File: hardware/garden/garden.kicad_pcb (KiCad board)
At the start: 4 copper layers, 53.3 x 83.8 mm, 53 parts, among them J1 CONN_01X40, J2 CONN_01X08, J3 CONN_01X06, J4 CONN_01X10, J5 CONN_01X08, J7 Micro_SD_Card_CD, J8 CONN_01X13, J9 CONN_01X06, M1 ESP-11, M2 CONN_01X01, M3 CONN_01X01, M4 CONN_01X01, M5 CONN_01X01, P1 USB_OTG, Q1 Q_NMOS_GSD, SW1 RESET, SW2 BOOT, U1 AZ1117-3.3, U2 STM32F745ZETx, U3 IS42S16160G, Y1 12MHz

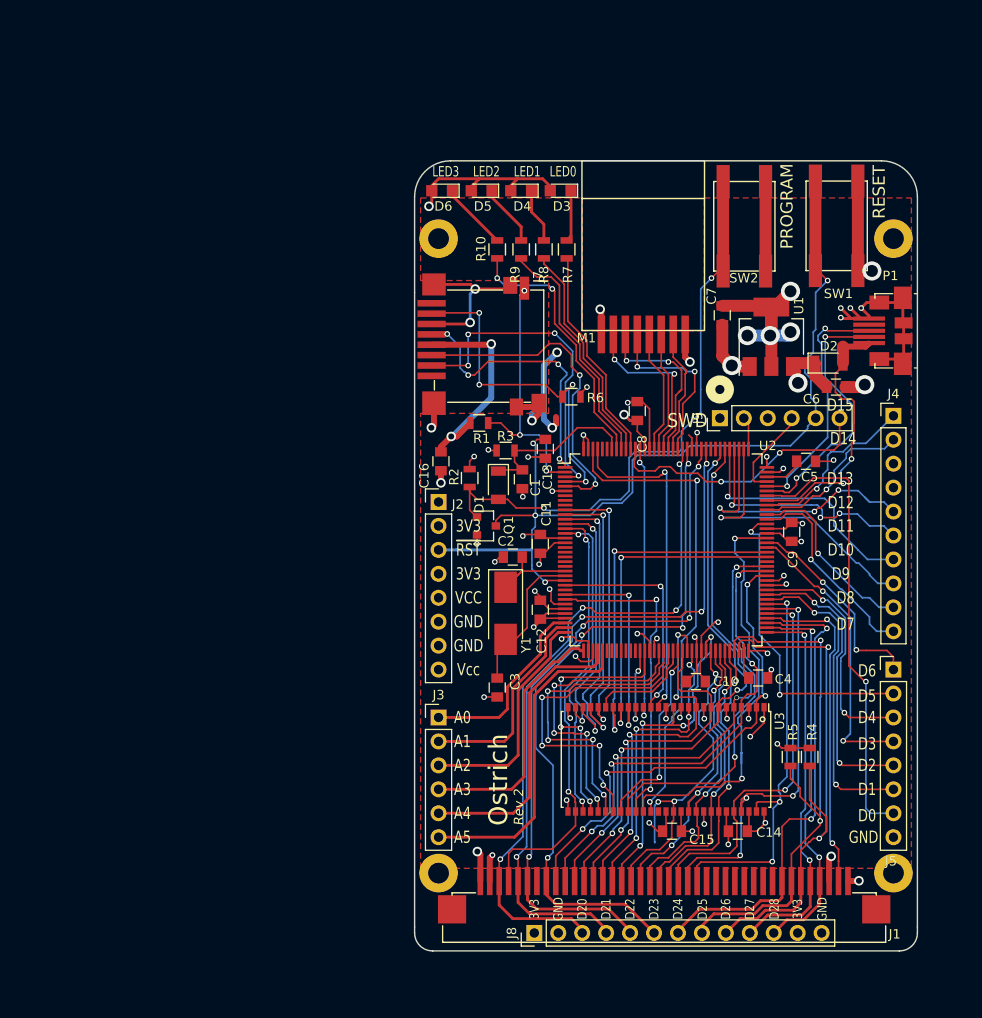
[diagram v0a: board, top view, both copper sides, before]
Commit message: Designed garden controller
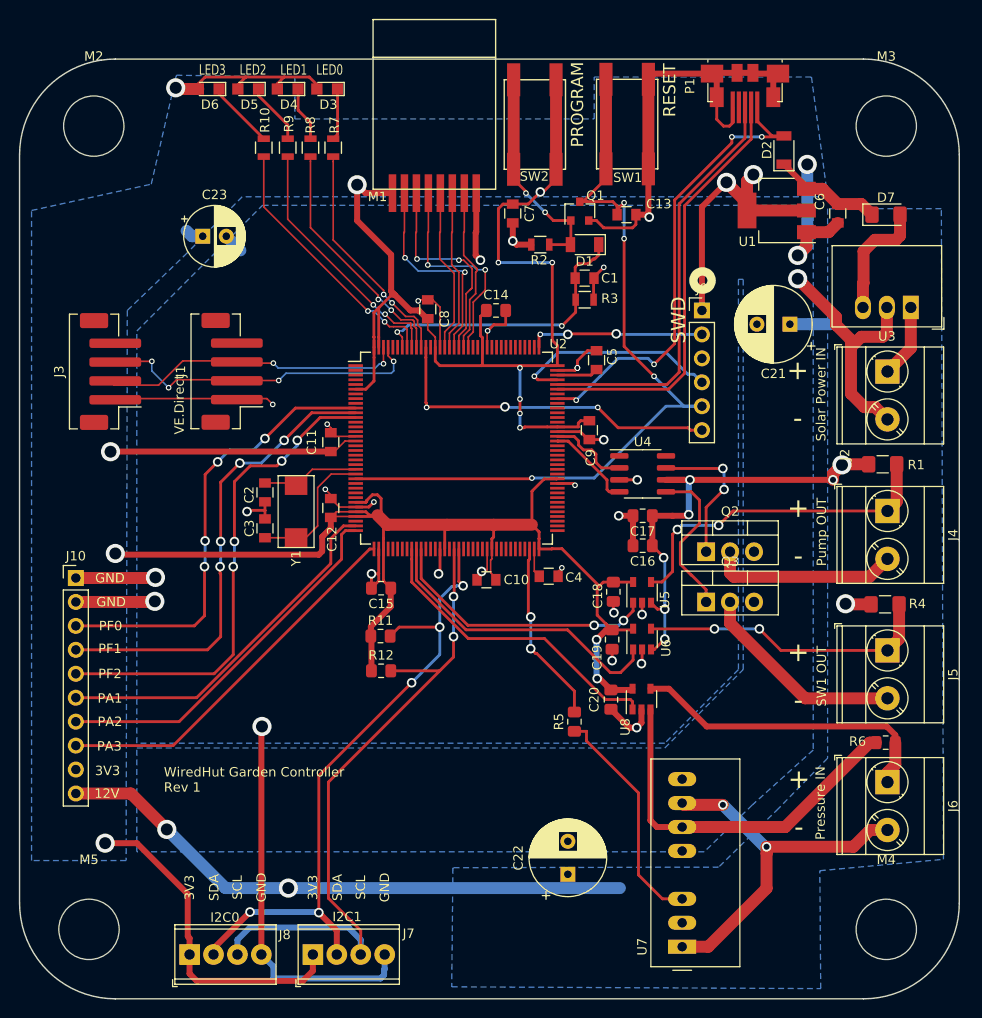
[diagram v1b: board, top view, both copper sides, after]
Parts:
- added C17: 1uF, Capacitor_SMD:C_0805_2012Metric_Pad1.15x1.40mm_HandSolder, F.Cu at (122.0, 98.0)
- added C18: 0.1uF, Capacitor_SMD:C_0805_2012Metric_Pad1.15x1.40mm_HandSolder, F.Cu at (118.9, 106.0)
- added C19: 0.1uF, Capacitor_SMD:C_0805_2012Metric_Pad1.15x1.40mm_HandSolder, F.Cu at (118.7, 111.1)
- added C20: 0.1uF, Capacitor_SMD:C_0805_2012Metric_Pad1.15x1.40mm_HandSolder, F.Cu at (118.6, 117.5)
- added C21: 220uF, Capacitor_THT:CP_Radial_D8.0mm_P3.50mm, F.Cu at (137.6, 77.7)
- added C22: 220uF, Capacitor_THT:CP_Radial_D8.0mm_P3.50mm, F.Cu at (114.0, 136.0)
- added C23: 22uF, Capacitor_THT:CP_Radial_D6.3mm_P2.50mm, F.Cu at (75.3, 68.3)
- added D7: D_Schottky, Diode_SMD:D_1206_3216Metric_Pad1.42x1.75mm_HandSolder, F.Cu at (147.8, 66.0)
- added J10: CONN_01X10, Connector_PinHeader_2.54mm:PinHeader_1x10_P2.54mm_Vertical, F.Cu at (61.8, 104.6)
- added J6: CONN_01X02, TerminalBlock_Phoenix:TerminalBlock_Phoenix_MKDS-3-2-5.08_1x02_P5.08mm_Horizontal, F.Cu at (148.0, 126.2)
- added Q2: Q_NMOS_GDS, Package_TO_SOT_THT:TO-220-3_Vertical, F.Cu at (128.7, 101.8)
- added Q3: Q_NMOS_GDS, Package_TO_SOT_THT:TO-220-3_Vertical, F.Cu at (128.7, 107.1)
- added R11: 1kR, Resistor_SMD:R_0805_2012Metric_Pad1.15x1.40mm_HandSolder, F.Cu at (94.2, 110.7)
- added R12: 1kR, Resistor_SMD:R_0805_2012Metric_Pad1.15x1.40mm_HandSolder, F.Cu at (94.2, 114.4)
- added U4: MIC4427, Package_SO:SOIC-8_3.9x4.9mm_P1.27mm, F.Cu at (122.0, 93.5)
- added U5: INA193, Package_TO_SOT_SMD:SOT-23-5, F.Cu at (121.9, 106.1)
- added U6: INA193, Package_TO_SOT_SMD:SOT-23-5, F.Cu at (121.9, 111.1)
- added U7: TEC2-1215WI, Converter_DCDC:Converter_DCDC_TRACO_TMR-xxxx_THT, F.Cu at (126.2, 143.7)
- added U8: INA193, Package_TO_SOT_SMD:SOT-23-5, F.Cu at (121.9, 117.4)
- C14: footprint Capacitors_SMD:C_0805 -> Capacitor_SMD:C_0805_2012Metric_Pad1.15x1.40mm_HandSolder
- C15, C16: value 10uF -> 0.1uF; footprint Capacitors_SMD:C_0805 -> Capacitor_SMD:C_0805_2012Metric_Pad1.15x1.40mm_HandSolder
- J1: value CONN_01X40 -> CONN_01X04; footprint ER-CON40HB-2:ER-CON40HB-2 -> Connector_JST:JST_PH_B4B-PH-SM4-TB_1x04-1MP_P2.00mm_Vertical
- J2, J5: value CONN_01X08 -> CONN_01X02; footprint Pin_Headers:Pin_Header_Straight_1x08_Pitch2.54mm -> TerminalBlock_Phoenix:TerminalBlock_Phoenix_MKDS-3-2-5.08_1x02_P5.08mm_Horizontal
- J3: value CONN_01X06 -> CONN_01X04; footprint Pin_Headers:Pin_Header_Straight_1x06_Pitch2.54mm -> Connector_JST:JST_PH_B4B-PH-SM4-TB_1x04-1MP_P2.00mm_Vertical
- J4: value CONN_01X10 -> CONN_01X02; footprint Connector_PinHeader_2.54mm:PinHeader_1x10_P2.54mm_Vertical -> TerminalBlock_Phoenix:TerminalBlock_Phoenix_MKDS-3-2-5.08_1x02_P5.08mm_Horizontal
- J7: value Micro_SD_Card_CD -> CONN_01X04; footprint Amphenol:Amphenol_1140084168 -> TerminalBlock_Phoenix:TerminalBlock_Phoenix_MPT-0,5-4-2.54_1x04_P2.54mm_Horizontal
- J8: value CONN_01X13 -> CONN_01X04; footprint Pin_Headers:Pin_Header_Straight_1x13_Pitch2.54mm -> TerminalBlock_Phoenix:TerminalBlock_Phoenix_MPT-0,5-4-2.54_1x04_P2.54mm_Horizontal
- M2, M3, M4, M5: footprint Mechanical:M2_HOLE -> MountingHole:MountingHole_6.4mm_M6
- R1, R4: value 10KR -> 10mR; footprint Resistors_SMD:R_0805 -> Resistor_SMD:R_1206_3216Metric_Pad1.42x1.75mm_HandSolder
- R5: value 10KR -> 1kR; footprint Resistors_SMD:R_0805 -> Resistor_SMD:R_0805_2012Metric_Pad1.15x1.40mm_HandSolder
- R6: value 10KR -> 6.8R; footprint Resistors_SMD:R_0805 -> Resistor_SMD:R_0805_2012Metric_Pad1.15x1.40mm_HandSolder
- U1: footprint SOT-223 -> Package_TO_SOT_SMD:SOT-223
- U3: value IS42S16160G -> R-78B5.0-2.0; footprint TSOPII:TSOPII-54_10.16x22.22mm-Pitch0.8mm -> Converter_DCDC:Converter_DCDC_RECOM_R-78B-2.0_THT
- moved J1 85.4 mm to (78.4, 82.7), turned to 90 degrees
- moved J7 70.5 mm to (87.0, 144.5), turned to 0 degrees
- moved C14 60.9 mm to (106.4, 76.2)
- moved U3 54.5 mm to (150.4, 75.9), turned to 180 degrees
- moved J3 50.6 mm to (65.5, 82.7), turned to 90 degrees
- moved J2 49.6 mm to (148.0, 82.7), turned to 270 degrees
- moved R6 49.6 mm to (147.8, 122.0)
- moved R1 43.0 mm to (147.4, 92.5)
- moved C15 40.2 mm to (94.2, 105.7)
- moved M2 38.5 mm to (63.8, 56.6)
- moved M5 37.6 mm to (63.2, 141.9)
- moved J8 36.6 mm to (73.9, 144.5), turned to 0 degrees
- moved Q1 34.8 mm to (115.3, 65.7), turned to 90 degrees
- moved P1 30.3 mm to (132.8, 52.3), turned to 270 degrees
- moved C3 29.9 mm to (81.9, 99.3), turned to 90 degrees
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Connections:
- net /PA9 renamed /Vusb
- C16 pad 1: +3V3 -> +12V
- J1 pad 2: /LCD_BL -> /VD_RX
- J1 pad 3: GND -> /VD_TX
- J1 pad 4: /TOUCH_WAKE -> (no net)
- J2 pad 1: Net-(J2-Pad1) -> +12V
- J2 pad 2: +3V3 -> GND
- J3 pad 1: /PA0 -> GND
- J3 pad 2: /PA1 -> /VD_TX
- J3 pad 3: /PA2 -> /VD_RX
- J3 pad 4: /PA3 -> (no net)
- J4 pad 1: /PA8 -> Net-(J4-Pad1)
- J4 pad 2: /PC9 -> Net-(J4-Pad2)
- J5 pad 1: /PG7 -> Net-(J5-Pad1)
- J5 pad 2: /PC6 -> Net-(J5-Pad2)
- J7 pad 1: Net-(J7-Pad1) -> +3V3
- J7 pad 2: /SD_CS -> /SDA
- J7 pad 3: /SD_MOSI -> /SCL
- J7 pad 4: +3V3 -> GND
- J8 pad 2: GND -> /SDA
- J8 pad 3: /~LCD_CS -> /SCL
- J8 pad 4: /~LCD_RD -> GND
- M2 pad 1: Net-(M2-Pad1) -> (no net)
- M3 pad 1: Net-(M3-Pad1) -> (no net)
- M4 pad 1: Net-(M4-Pad1) -> (no net)
- M5 pad 1: Net-(M5-Pad1) -> (no net)
- P1 pad 4: Net-(P1-Pad4) -> (no net)
- R1 pad 1: +3V3 -> +12V
- R1 pad 2: /SD_CD -> Net-(J4-Pad1)
- R4 pad 1: +3V3 -> +12V
- R4 pad 2: /TOUCH_SDA -> Net-(J5-Pad1)
- R5 pad 1: +3V3 -> Net-(R5-Pad1)
- R5 pad 2: /TOUCH_SCL -> /PRESSURE_PWR
- R6 pad 1: +3V3 -> Net-(J6-Pad1)
- R6 pad 2: /SD_MISO -> Net-(R6-Pad2)
- U2 pad 1: /SD_SCLK -> (no net)
- U2 pad 10: /A0 -> /PF0
- U2 pad 100: /PA8 -> (no net)
- U2 pad 102: /PA10 -> (no net)
- U2 pad 11: /A1 -> /PF1
- U2 pad 110: /PA15 -> (no net)
- U2 pad 111: /PC10 -> (no net)
- U2 pad 112: /PC11 -> (no net)
- U2 pad 113: /PC12 -> (no net)
- U2 pad 114: /D2 -> (no net)
- U2 pad 115: /D3 -> (no net)
- U2 pad 116: Net-(U2-Pad116) -> (no net)
- U2 pad 117: Net-(U2-Pad117) -> (no net)
- U2 pad 118: /~LCD_RD -> (no net)
- U2 pad 119: /~LCD_WR -> (no net)
- U2 pad 12: /A2 -> /PF2
- U2 pad 122: /LCD_TE -> (no net)
- U2 pad 123: /~LCD_CS -> (no net)
- U2 pad 13: /A3 -> (no net)
- U2 pad 132: /SDNCAS -> (no net)
- U2 pad 139: Net-(U2-Pad139) -> (no net)
- U2 pad 14: /A4 -> (no net)
- U2 pad 140: Net-(U2-Pad140) -> (no net)
- U2 pad 141: /NBL0 -> /VD_RX
- U2 pad 142: /NBL1 -> /VD_TX
- U2 pad 15: /A5 -> (no net)
- U2 pad 18: Net-(U2-Pad18) -> (no net)
- U2 pad 19: Net-(U2-Pad19) -> (no net)
- U2 pad 2: /SD_CD -> (no net)
- U2 pad 20: Net-(U2-Pad20) -> (no net)
- U2 pad 21: Net-(U2-Pad21) -> (no net)
- U2 pad 22: Net-(U2-Pad22) -> (no net)
- U2 pad 26: /SDNWE -> (no net)
- U2 pad 27: Net-(U2-Pad27) -> (no net)
- U2 pad 28: /SDNE0 -> (no net)
- U2 pad 29: /SDCKE0 -> (no net)
- U2 pad 3: /SD_CS -> (no net)
- U2 pad 34: /PA0 -> (no net)
- U2 pad 4: /SD_MISO -> (no net)
- U2 pad 40: /PA4 -> (no net)
- U2 pad 41: /PA5 -> (no net)
- U2 pad 42: Net-(U2-Pad42) -> (no net)
- U2 pad 43: /PA7 -> (no net)
- U2 pad 44: Net-(U2-Pad44) -> (no net)
- U2 pad 45: Net-(U2-Pad45) -> /PRESSURE_CUR
- U2 pad 46: Net-(U2-Pad46) -> /SW1_CUR
- U2 pad 47: Net-(U2-Pad47) -> /SW0_CUR
- U2 pad 48: Net-(U2-Pad48) -> (no net)
- U2 pad 49: /SDNRAS -> (no net)
- U2 pad 5: /SD_MOSI -> (no net)
- U2 pad 50: /A6 -> (no net)
- U2 pad 53: /A7 -> (no net)
- U2 pad 54: /A8 -> /SCL
- U2 pad 55: /A9 -> /SDA
- U2 pad 56: /A10 -> (no net)
- U2 pad 57: /A11 -> (no net)
- U2 pad 58: /D4 -> (no net)
- U2 pad 59: /D5 -> (no net)
- U2 pad 60: /D6 -> (no net)
- U2 pad 63: /D7 -> (no net)
- U2 pad 64: /D8 -> (no net)
- U2 pad 65: /D9 -> (no net)
- U2 pad 66: /D10 -> (no net)
- U2 pad 67: /D11 -> (no net)
- U2 pad 68: /D12 -> (no net)
- U2 pad 69: /TOUCH_SCL -> (no net)
- U2 pad 7: Net-(U2-Pad7) -> (no net)
- U2 pad 70: /TOUCH_SDA -> /PRESSURE_PWR
- U2 pad 73: /TOUCH_INT -> (no net)
- U2 pad 74: /TOUCH_WAKE -> (no net)
- U2 pad 75: /TOUCH_RESET -> (no net)
- U2 pad 76: /LCD_BL -> (no net)
- U2 pad 77: /D13 -> (no net)
- U2 pad 78: /D14 -> (no net)
- U2 pad 79: /D15 -> (no net)
- U2 pad 8: Net-(U2-Pad8) -> (no net)
- U2 pad 80: /PD11 -> (no net)
- U2 pad 81: /PD12 -> (no net)
- U2 pad 82: /PD13 -> (no net)
- U2 pad 85: /D0 -> (no net)
- U2 pad 86: /D1 -> (no net)
- U2 pad 87: /A12 -> (no net)
- U2 pad 88: Net-(U2-Pad88) -> (no net)
- U2 pad 89: /BA0 -> (no net)
- U2 pad 9: Net-(U2-Pad9) -> (no net)
- U2 pad 90: /BA1 -> (no net)
- U2 pad 91: /PG6 -> (no net)
- U2 pad 92: /PG7 -> /SW1_SIG
- U2 pad 93: /SDCLK -> /SW0_SIG
- U2 pad 96: /PC6 -> (no net)
- U2 pad 97: /PC7 -> (no net)
- U2 pad 98: /PC8 -> (no net)
- U2 pad 99: /PC9 -> (no net)
- U3 pad 1: +3V3 -> +12V
- U3 pad 2: /D0 -> GND
- U3 pad 3: +3V3 -> Net-(D7-Pad2)
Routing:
- net +3V3: track 159.8 -> 354.3 mm, vias 33 -> 16
- net GND: track 145.8 -> 297.4 mm, vias 41 -> 34
- net +12V: track 0.00 -> 126.2 mm, vias 0 -> 10
- net VCC: track 116.1 -> 11.7 mm, vias 1 -> 0
- net /~LCD_RD: track 74.5 -> 0.00 mm, vias 4 -> 0
- net /~LCD_WR: track 74.3 -> 0.00 mm, vias 4 -> 0
- net /LCD_TE: track 74.2 -> 0.00 mm, vias 4 -> 0
- net /~LCD_CS: track 73.3 -> 0.00 mm, vias 4 -> 0
- net /SCL: track 0.00 -> 72.5 mm, vias 0 -> 2
- net /SDA: track 0.00 -> 70.1 mm, vias 0 -> 5
- net /D2: track 62.1 -> 0.00 mm, vias 4 -> 0
- net /D3: track 60.2 -> 0.00 mm, vias 4 -> 0
- net /TOUCH_SCL: track 58.1 -> 0.00 mm, vias 2 -> 0
- net /TOUCH_SDA: track 57.6 -> 0.00 mm, vias 2 -> 0
- net /D0: track 52.2 -> 0.00 mm, vias 4 -> 0
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- added copper zone on B.Cu, net +12V
- added copper zone on B.Cu, net +3V3
- added copper zone on B.Cu, net GND
- removed copper zone on F.Cu, net +3V3
- removed copper zone on VDD, net +3V3
- removed copper zone on GND, net GND
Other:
- board size 53.3 x 83.8 mm -> 99.7 x 99.7 mm
- copper layers 4 -> 2
- rule via_min_size: 0.4 -> 0.45
- board text added: "+"
- board text added: "-"
- board text added: "12V"
- board text added: "I2C0"
- board text added: "I2C1"
- board text added: "PA1"
- board text added: "PA2"
- board text added: "PA3"
- board text added: "PF0"
- board text added: "PF1"
- board text added: "PF2"
- board text added: "Pressure IN"
- board text added: "Pump OUT"
- board text added: "SCL"
- board text added: "SDA"
- board text added: "SW1 OUT"
- board text added: "Solar Power IN"
- board text added: "VE.Direct"
- board text added: "WiredHut Garden Controller Rev 1"
- board text removed: "A0"
- board text removed: "A1"
- board text removed: "A2"
- board text removed: "A3"
- board text removed: "A4"
- board text removed: "A5"
- board text removed: "D0"
- board text removed: "D1"
- board text removed: "D10"
- board text removed: "D11"
- board text removed: "D12"
- board text removed: "D13"
- board text removed: "D14"
- board text removed: "D15"
- board text removed: "D2"
- board text removed: "D20"
- board text removed: "D21"
- board text removed: "D22"
- board text removed: "D23"
- board text removed: "D24"
- board text removed: "D25"
- board text removed: "D26"
- board text removed: "D27"
- board text removed: "D28"
- board text removed: "D3"
- board text removed: "D4"
- board text removed: "D5"
- board text removed: "D6"
- board text removed: "D7"
- board text removed: "D8"
- board text removed: "D9"
- board text removed: "Ostrich"
- board text removed: "Rev 2"
- board text removed: "VCC"
- board text removed: "Vcc"
- board text removed: "~RST"
